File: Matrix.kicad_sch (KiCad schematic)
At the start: 72 parts, among them SW1 SW_Push, SW10 SW_Push, SW11 SW_Push, SW12 SW_Push, SW13 SW_Push, SW14 SW_Push, SW15 SW_Push, SW16 SW_Push, SW17 SW_Push, SW18 SW_Push, SW2 SW_Push, SW3 SW_Push, SW4 SW_Push, SW5 SW_Push, SW6 SW_Push, SW7 SW_Push, SW8 SW_Push, SW9 SW_Push

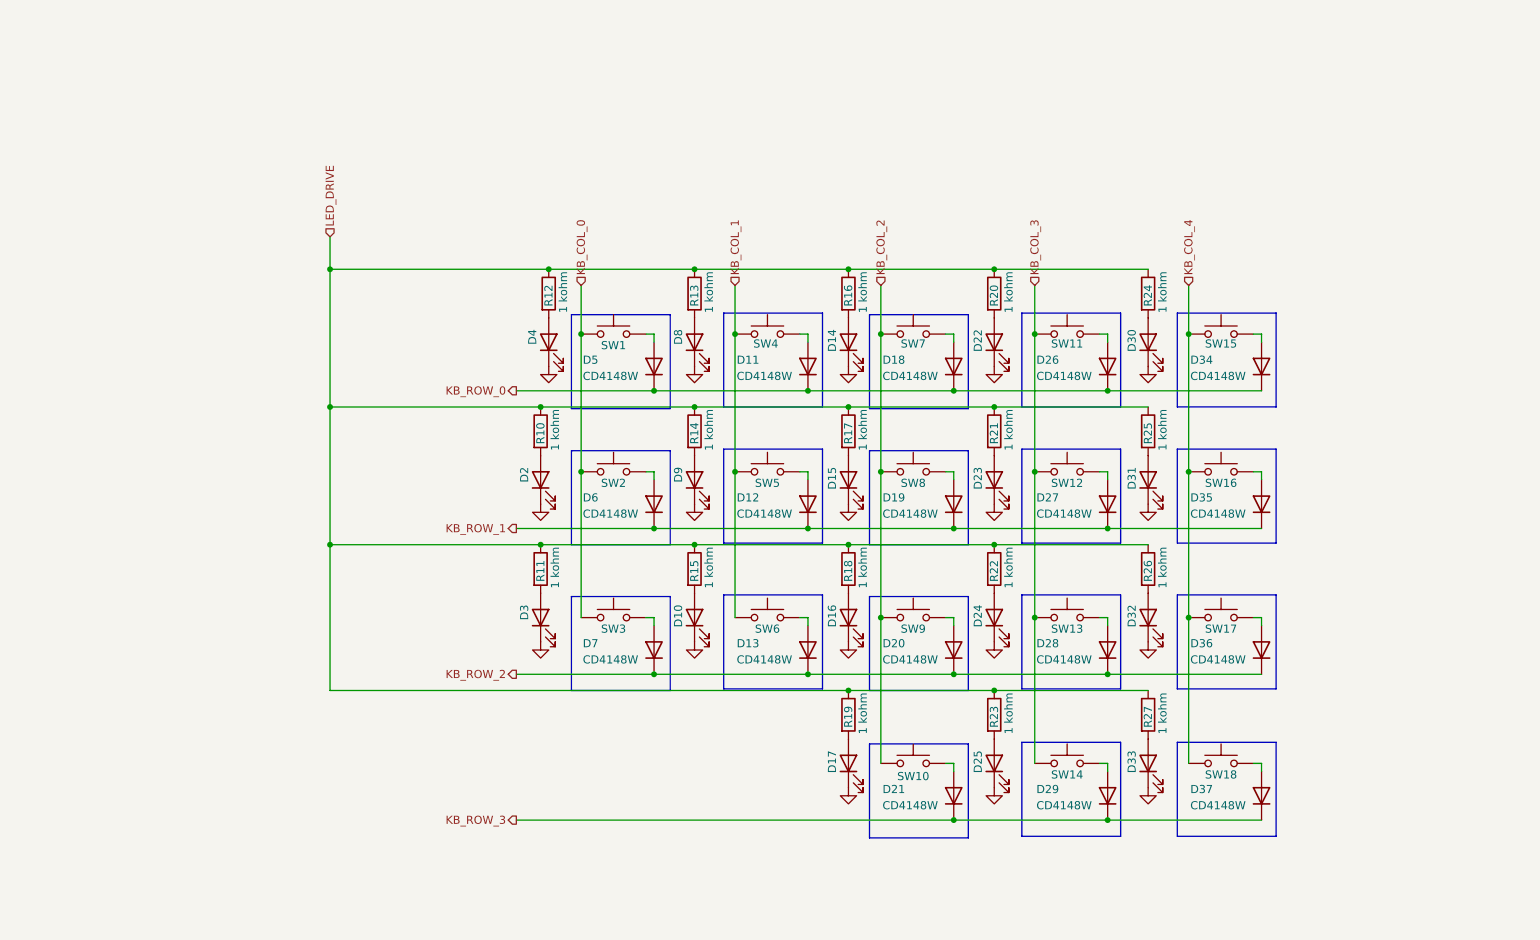
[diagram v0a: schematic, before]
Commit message: update power mgmt
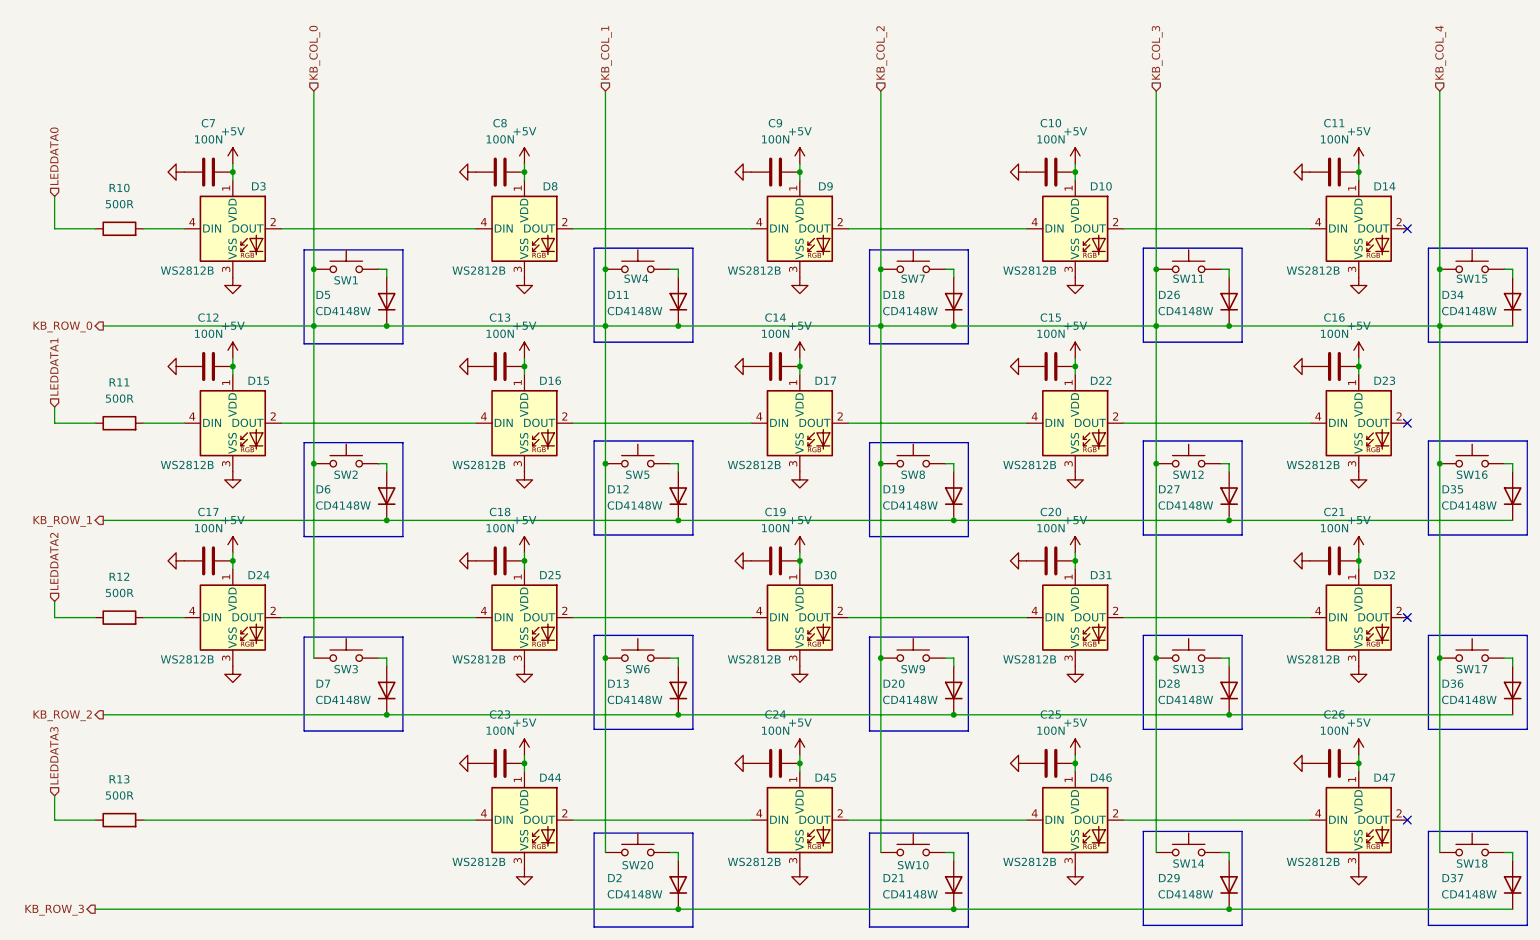
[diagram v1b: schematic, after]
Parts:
- removed D10, D14, D15, D16, D17, D2, D22, D23, D24, D25, D3, D30, D31, D32, D33, D4, D8, D9: LED, LED_SMD:LED_0603_1608Metric_Pad1.05x0.95mm_HandSolder, symbol Device:LED
- removed R10, R11, R12, R13, R14, R15, R16, R17, R18, R19, R20, R21, R22, R23, R24, R25, R26, R27: 1 kohm, Resistor_SMD:R_0603_1608Metric_Pad0.98x0.95mm_HandSolder, symbol #inventree:RC0603FR-071KL
- added C10, C11, C12, C13, C14, C15, C16, C17, C18, C19, C20, C21, C23, C24, C25, C26, C7, C8, C9: 100N, Capacitor_SMD:C_0603_1608Metric_Pad1.08x0.95mm_HandSolder, symbol Device:C
- added D10, D14, D15, D16, D17, D22, D23, D24, D25, D3, D30, D31, D32, D44, D45, D46, D47, D8, D9: WS2812B, LED_SMD:LED_WS2812_PLCC6_5.0x5.0mm_P1.6mm, symbol LED:WS2812B
- added D2: CD4148W, Diode_SMD:D_0805_2012Metric_Pad1.15x1.40mm_HandSolder, symbol Diode:CD4148W
- added R10, R11, R12, R13: 500R, Resistor_SMD:R_0603_1608Metric_Pad0.98x0.95mm_HandSolder, symbol Device:R
- added SW20: SW_Push, personal:Gateron_Milky_Yellow, symbol Switch:SW_Push
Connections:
- net KB_COL_1 is gone; now on net KB_COL_0: SW4.1, SW5.1, SW6.1
- net KB_COL_2 is gone; now on net KB_COL_0: SW10.1, SW7.1, SW8.1, SW9.1
- net KB_COL_3 is gone; now on net KB_COL_0: SW11.1, SW12.1, SW13.1, SW14.1
- net KB_COL_4 is gone; now on net KB_COL_0: SW15.1, SW16.1, SW17.1, SW18.1
- net KB_ROW_0 is gone; now on net KB_COL_0: D11.1 (K), D18.1 (K), D26.1 (K), D34.1 (K), D5.1 (K)
- net GND: now also C10.1, C11.1, C12.1, C13.1, C14.1, C15.1, C16.1, C17.1, C18.1, C19.1, C20.1, C21.1, C23.1, C24.1, C25.1, C26.1, C7.1, C8.1, C9.1, D10.3 (VSS), D14.3 (VSS), D15.3 (VSS), D16.3 (VSS), D17.3 (VSS), D22.3 (VSS), D23.3 (VSS), D24.3 (VSS), D25.3 (VSS), D3.3 (VSS), D30.3 (VSS), D31.3 (VSS), D32.3 (VSS), D44.3 (VSS), D45.3 (VSS), D46.3 (VSS), D47.3 (VSS), D8.3 (VSS), D9.3 (VSS)
- net KB_COL_0: now also SW20.1
- net KB_ROW_3: now also D2.1 (K)
- new net: D3.4 (DIN), R10.2
- new net: D24.4 (DIN), R12.2
- new net: D25.2 (DOUT), D30.4 (DIN)
- new net: D24.2 (DOUT), D25.4 (DIN)
- new net: D10.4 (DIN), D9.2 (DOUT)
- new net: D8.2 (DOUT), D9.4 (DIN)
- new net: D45.2 (DOUT), D46.4 (DIN)
- new net: D44.2 (DOUT), D45.4 (DIN)
- new net: D30.2 (DOUT), D31.4 (DIN)
- new net: D10.2 (DOUT), D14.4 (DIN)
- new net: D15.4 (DIN), R11.2
- new net: D3.2 (DOUT), D8.4 (DIN)
- new net: D16.2 (DOUT), D17.4 (DIN)
- new net: D15.2 (DOUT), D16.4 (DIN)
- new net: D31.2 (DOUT), D32.4 (DIN)
- new net: D22.2 (DOUT), D23.4 (DIN)
- new net: D17.2 (DOUT), D22.4 (DIN)
- new net: D46.2 (DOUT), D47.4 (DIN)
- new net: D44.4 (DIN), R13.2
- new net: D2.2 (A), SW20.2
- new net +5V: C10.2, C11.2, C12.2, C13.2, C14.2, C15.2, C16.2, C17.2, C18.2, C19.2, C20.2, C21.2, C23.2, C24.2, C25.2, C26.2, C7.2, C8.2, C9.2, D10.1 (VDD), D14.1 (VDD), D15.1 (VDD), D16.1 (VDD), D17.1 (VDD), D22.1 (VDD), D23.1 (VDD), D24.1 (VDD), D25.1 (VDD), D3.1 (VDD), D30.1 (VDD), D31.1 (VDD), D32.1 (VDD), D44.1 (VDD), D45.1 (VDD), D46.1 (VDD), D47.1 (VDD), D8.1 (VDD), D9.1 (VDD)
- new net LEDDATA0: R10.1
- new net LEDDATA1: R11.1
- new net LEDDATA2: R12.1
- new net LEDDATA3: R13.1
- no-connect marks 0 -> 4
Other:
- moved on the sheet: D11, D12, D13, D18, D19, D20, D21, D26, D27, D28, D29, D34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
